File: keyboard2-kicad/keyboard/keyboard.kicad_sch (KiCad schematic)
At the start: 449 parts, among them J1 DC-005, J2 TYPE-C-31-M-12, J3 Touchscreen, J4 Touchscreen, M1 Motor_Servo, M10 Motor_Servo, M2 Motor_Servo, M3 Motor_Servo, M4 Motor_Servo, M5 Motor_Servo, M6 Motor_Servo, M7 Motor_Servo, M8 Motor_Servo, M9 Motor_Servo, SW1 Esc, SW10 F9, SW100 Enter, SW101 RotaryEncoder, SW11 F10, SW12 F11, SW13 F12, SW14 DEL, SW15 HOME, SW16 END, SW17 PGUP, SW18 PGDN, SW19 INS, SW2 F1, SW20 TILDE, SW21 1, SW22 2, SW23 3, SW24 4, SW25 5, SW26 6, SW27 7, SW28 8, SW29 9, SW3 F2, SW30 0, SW31 -, SW32 =, SW33 BKSP, SW34 Num, SW35 /, SW36 *, SW37 -, SW38 Tab, SW39 Q, SW4 F3, SW40 W, SW41 E, SW42 R, SW43 T, SW44 Y, SW45 U, SW46 I, SW47 O, SW48 P, SW49 [, SW5 F4, SW50 ], SW51 \, SW52 7, SW53 8, SW54 9, SW55 Caps, SW56 A, SW57 S, SW58 D, SW59 F, SW6 F5, SW60 G, SW61 H, SW62 J, SW63 K, SW64 L, SW65 ;, SW66 ", SW67 Enter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

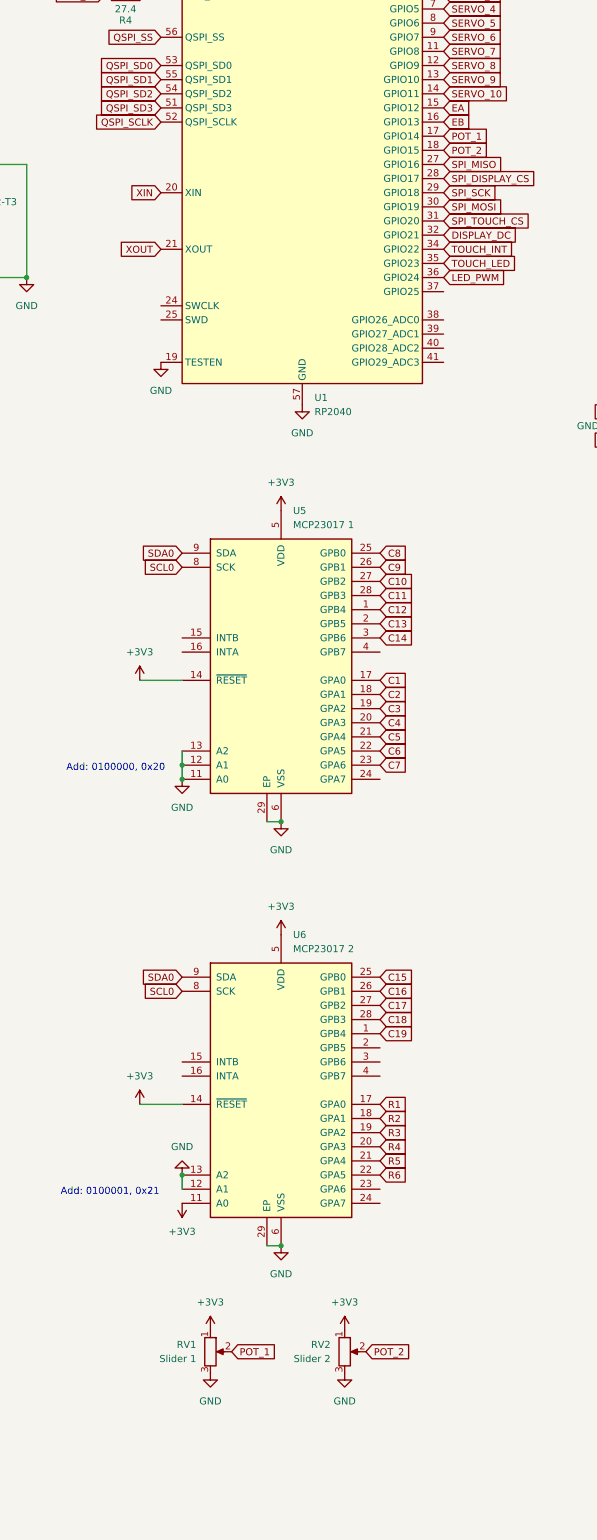
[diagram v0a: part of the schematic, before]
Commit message: yeah, just everything
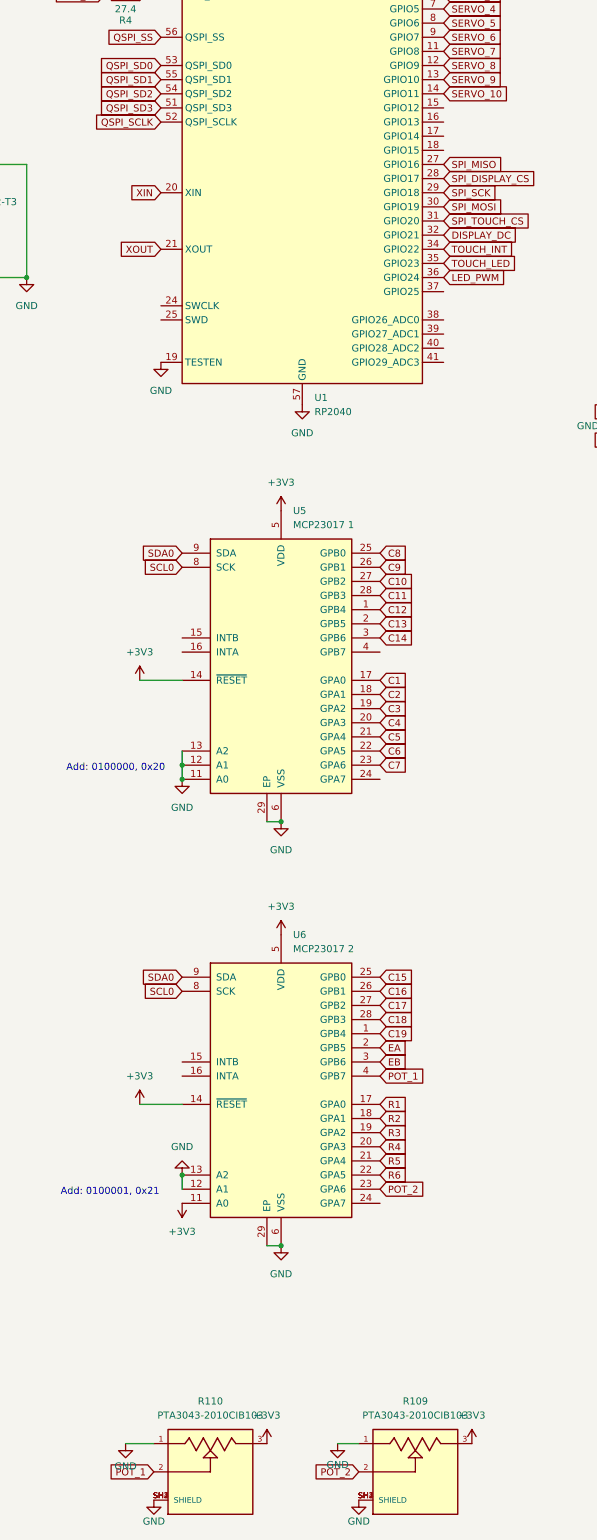
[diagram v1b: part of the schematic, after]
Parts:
- removed RV1: Slider 1, symbol Device:R_Potentiometer
- removed RV2: Slider 2, symbol Device:R_Potentiometer
- added R109, R110: PTA3043-2010CIB103, PTA3043-2010CIB103:TRIM_PTA3043-2010CIB103, symbol PTA3043-2010CIB103:PTA3043-2010CIB103
- SW101: footprint (none) -> EC10E1220501:TRIM_EC10E1220501
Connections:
- net +3V3: now also R109.3, R110.3
- net EA: now also U6.2 (GPB5); no longer U1.15 (GPIO12)
- net EB: now also U6.3 (GPB6); no longer U1.16 (GPIO13)
- net GND: now also R109.1, R109.SH1 (SHIELD), R109.SH2 (SHIELD), R109.SH3 (SHIELD), R109.SH4 (SHIELD), R110.1, R110.SH1 (SHIELD), R110.SH2 (SHIELD), R110.SH3 (SHIELD), R110.SH4 (SHIELD)
- net POT_1: now also U6.4 (GPB7), R110.2; no longer U1.17 (GPIO14)
- net POT_2: now also U6.23 (GPA6), R109.2; no longer U1.18 (GPIO15)
